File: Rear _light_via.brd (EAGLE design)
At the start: 59.8 x 72.7 mm, 9 parts

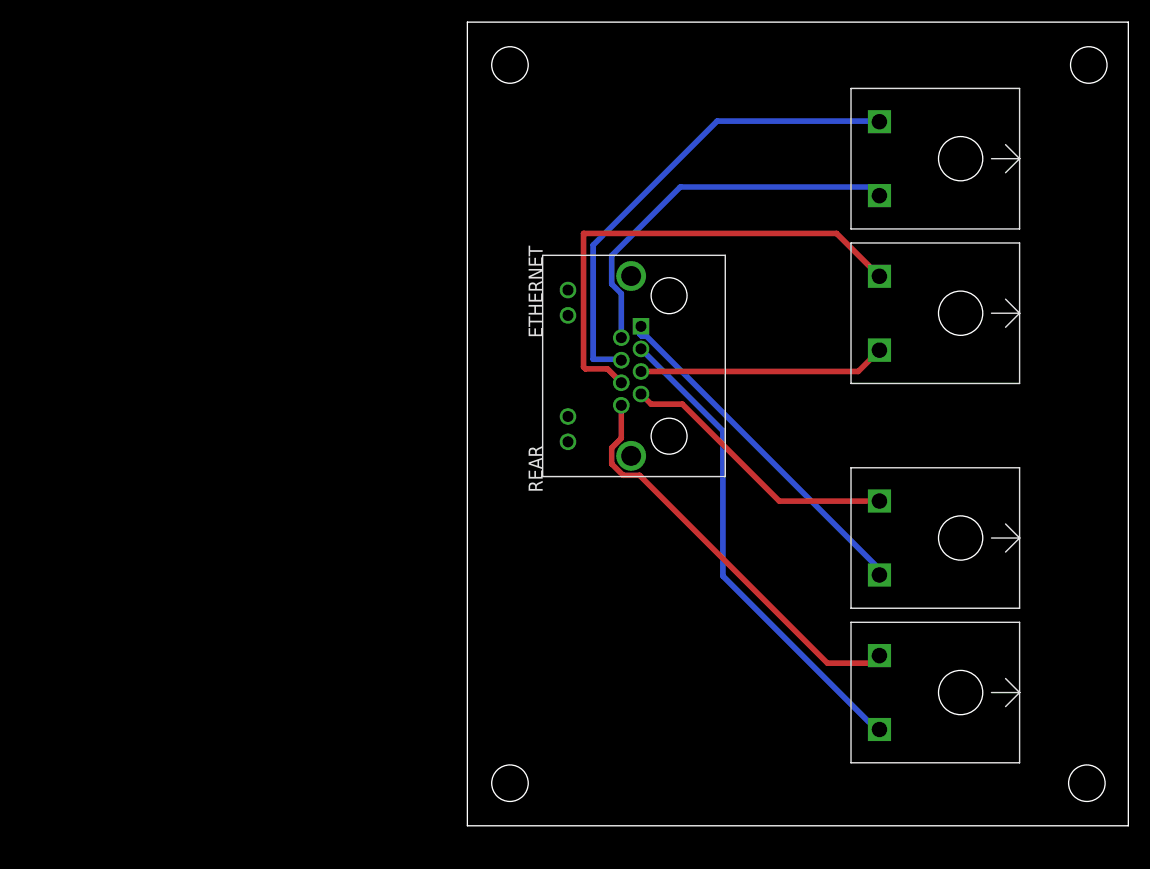
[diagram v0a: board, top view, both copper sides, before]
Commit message: via gerbers generated
via boards completed and gerbers generated
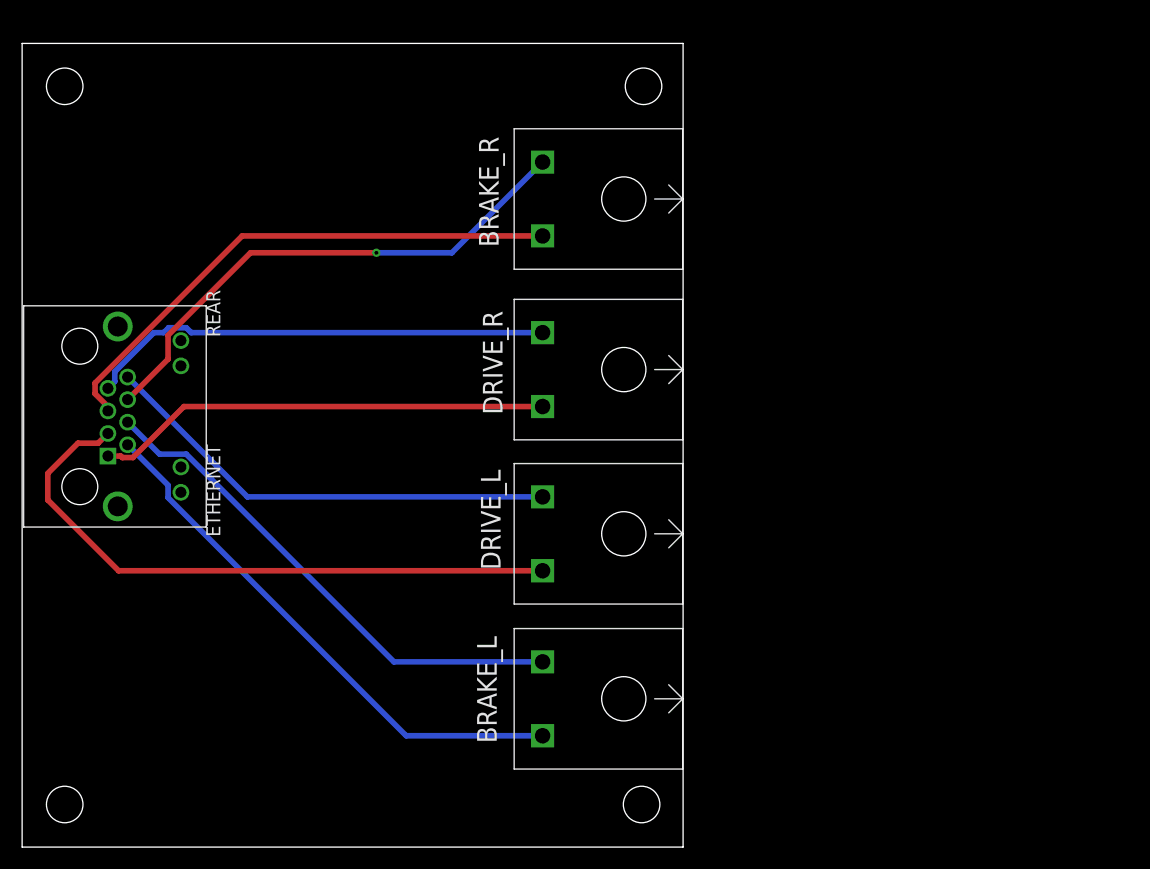
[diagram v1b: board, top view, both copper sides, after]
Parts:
- moved L_SIG 57.5 mm to (59.7, 13.4)
- moved REAR 53.5 mm to (5.21, 38.9), turned to 270 degrees
- moved H1 40.3 mm to (3.85, 3.85)
- moved H2 40.3 mm to (56.0, 3.85)
- moved H3 40.3 mm to (3.85, 68.8)
- moved H4 40.3 mm to (56.2, 68.8)
- moved L_DRIVE 34.0 mm to (59.7, 43.2)
- moved T_DRIVE 33.7 mm to (59.7, 28.3)
- moved R_SIG 32.2 mm to (59.7, 58.6)
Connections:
- net N$4 renamed BRAKE_L
- net N$5 renamed DRIVE_R
- net N$6 renamed BRAKE_R
- net N$8 renamed DRIVE_L
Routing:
- net N$3: track 23.1 -> 49.0 mm
- net DRIVE_R: track 25.6 -> 42.3 mm
- net N$2: track 35.7 -> 49.1 mm
- net N$7: track 43.5 -> 56.7 mm
- net N$1: track 32.3 -> 41.3 mm
- net DRIVE_L: track 37.6 -> 42.0 mm
- net BRAKE_R: track 44.8 -> 47.7 mm, vias 0 -> 1
- net BRAKE_L: track 45.5 -> 46.5 mm
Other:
- board text added: "BRAKE_L"
- board text added: "BRAKE_R"
- board text added: "DRIVE_L"
- board text added: "DRIVE_R"
